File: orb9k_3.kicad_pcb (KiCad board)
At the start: 2 copper layers, 49.3 x 33 mm, 14 parts, among them IC2 MAX3232, J1 DB9-PowerDTRRTS, U2 SeeeduinoXIAO, U4 TC1240A

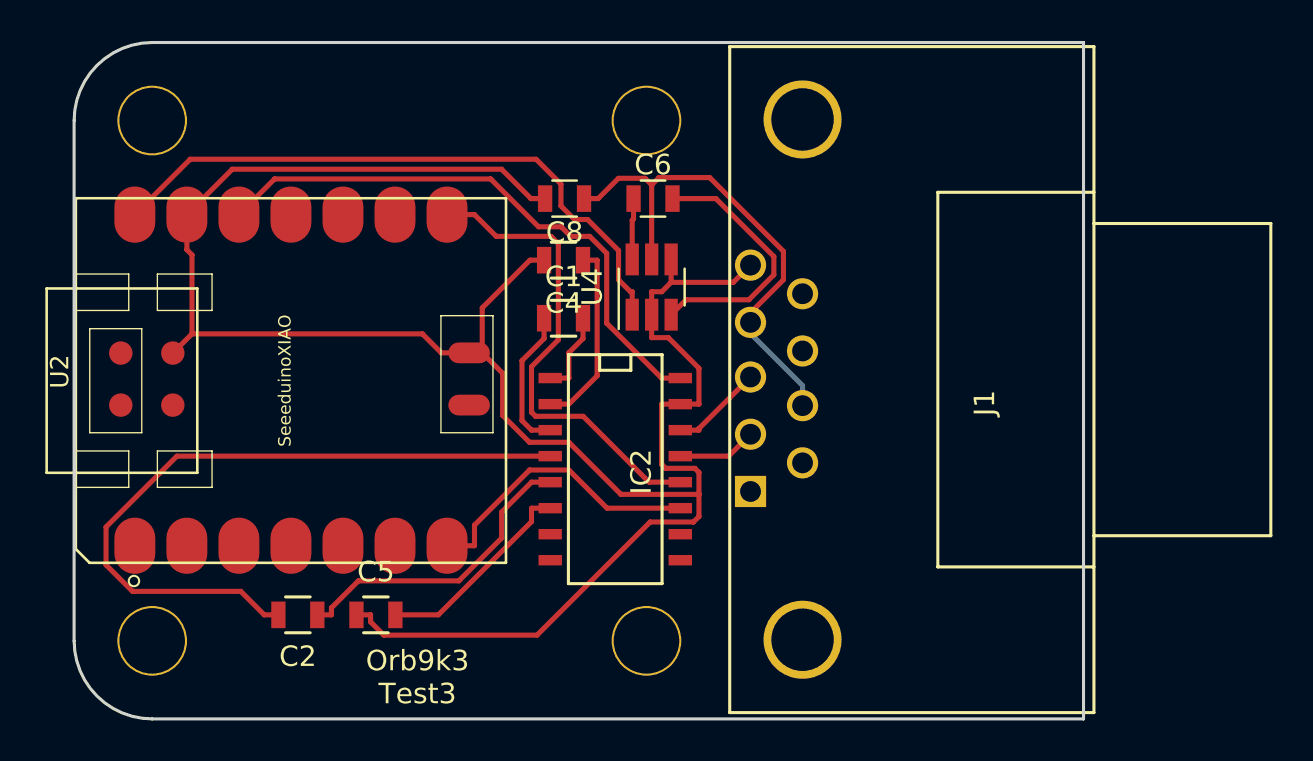
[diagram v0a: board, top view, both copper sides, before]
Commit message: Updates to orb9k_3
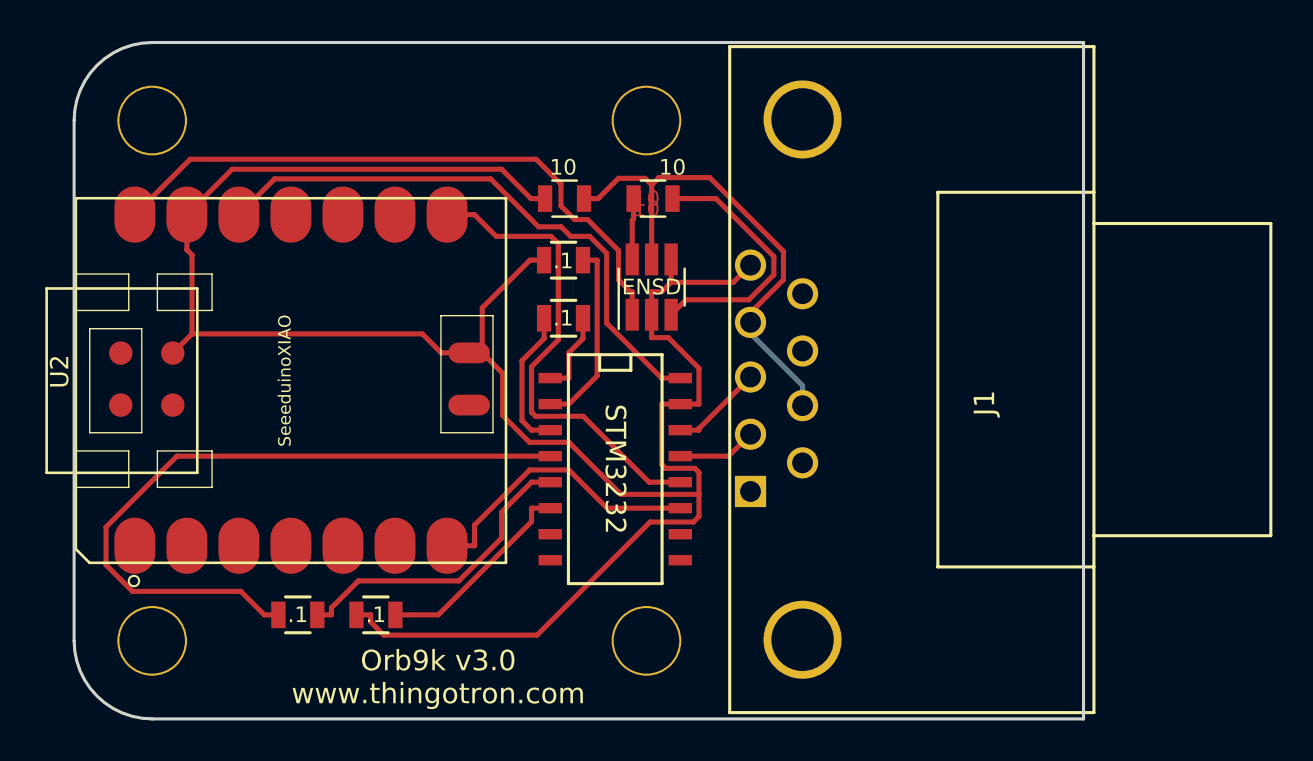
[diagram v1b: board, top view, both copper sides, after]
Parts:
- renumbered C1 to .1, C2 to .1, C4 to .1, C5 to .1, C8 to 10, C6 to 10, U4 to ENSD, IC2 to STM3232
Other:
- board text added: "10"
- board text added: "Orb9k v3.0 www.thingotron.com"
- board text removed: "Orb9k3 Test3"
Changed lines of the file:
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@@
   (general
     (thickness 1.6)
-    (drawings 8)
+    (drawings 10)
     (tracks 146)
     (zones 0)
@@
     (0 F.Cu signal)
     (31 B.Cu signal)
-    (32 B.Adhes user)
-    (33 F.Adhes user)
+    (32 B.Adhes user hide)
+    (33 F.Adhes user hide)
     (34 B.Paste user)
     (35 F.Paste user)
@@
     (47 F.CrtYd user)
     (48 B.Fab user)
-    (49 F.Fab user)
+    (49 F.Fab user hide)
   )
   (setup
@@
     (visible_elements 7FFFFFFF)
     (pcbplotparams
-      (layerselection 0x010f8_80000001)
+      (layerselection 0x010f8_ffffffff)
       (usegerberextensions true)
       (usegerberattributes false)
@@
       (drillshape 0)
       (scaleselection 1)
-      (outputdirectory "../proto_orders/20170102/"))
+      (outputdirectory "../proto_orders/20200509/gerbers"))
   )
   (net 0 "")
@@
     (tags "resistor 0805")
     (attr smd)
-    (fp_text reference C1 (at 0 2.032 180) (layer F.SilkS)
-      (effects (font (size 1 1) (thickness 0.15)))
+    (fp_text reference .1 (at 0.016 2.794 180) (layer F.SilkS)
+      (effects (font (size 0.762 0.762) (thickness 0.1524)))
     )
     (fp_text value 0.1uf (at 0 2.1 180) (layer F.Fab)
@@
     (tags "resistor 0805")
     (attr smd)
-    (fp_text reference C2 (at 0 2.032 180) (layer F.SilkS)
-      (effects (font (size 1 1) (thickness 0.15)))
+    (fp_text reference .1 (at 0 0 180) (layer F.SilkS)
+      (effects (font (size 0.762 0.762) (thickness 0.1524)))
     )
     (fp_text value 0.1uf (at 0 2.1 180) (layer F.Fab)
@@
     (tags "resistor 0805")
     (attr smd)
-    (fp_text reference C4 (at 0 -2.1 180) (layer F.SilkS)
-      (effects (font (size 1 1) (thickness 0.15)))
+    (fp_text reference .1 (at 0.016 -2.8365 180) (layer F.SilkS)
+      (effects (font (size 0.762 0.762) (thickness 0.1524)))
     )
     (fp_text value 0.1uf (at 0 2.1 180) (layer F.Fab)
@@
     (tags "resistor 0805")
     (attr smd)
-    (fp_text reference C5 (at 0 -2.1) (layer F.SilkS)
-      (effects (font (size 1 1) (thickness 0.15)))
+    (fp_text reference .1 (at 0 0) (layer F.SilkS)
+      (effects (font (size 0.762 0.762) (thickness 0.1524)))
     )
     (fp_text value 0.1uf (at -0.508 -2.032) (layer F.Fab)
@@
     (tags "CMS SOJ")
     (attr smd)
-    (fp_text reference IC2 (at 0.127 -1.27 270) (layer F.SilkS)
+    (fp_text reference STM3232 (at 0 0 270 unlocked) (layer F.SilkS)
       (effects (font (size 1 1) (thickness 0.15)))
     )
@@
     (tags "resistor 0805")
     (attr smd)
-    (fp_text reference C8 (at 0 -1.65) (layer F.SilkS)
-      (effects (font (size 1 1) (thickness 0.15)))
+    (fp_text reference 10 (at 0.066 1.524) (layer F.SilkS)
+      (effects (font (size 0.762 0.762) (thickness 0.1524)))
     )
     (fp_text value 10uf (at 0 1.75) (layer F.Fab)
@@
     (tags "SOT-23-6 Handsoldering")
     (attr smd)
-    (fp_text reference U4 (at 0 -2.9 90) (layer F.SilkS)
-      (effects (font (size 1 1) (thickness 0.15)))
+    (fp_text reference ENSD (at 0 0 180) (layer F.SilkS)
+      (effects (font (size 0.762 0.762) (thickness 0.1524)))
     )
     (fp_text value TC1240A (at 0 2.9 90) (layer F.Fab)
@@
     (tags "resistor 0805")
     (attr smd)
-    (fp_text reference C6 (at 0 -1.65) (layer F.SilkS)
-      (effects (font (size 1 1) (thickness 0.15)))
+    (fp_text reference 10 (at 0.95 -1.524) (layer F.SilkS)
+      (effects (font (size 0.762 0.762) (thickness 0.15)))
     )
     (fp_text value 10uf (at 0 1.75) (layer F.Fab)
@@
     )
   )
-  (gr_text "Orb9k3\nTest3" (at 61.764 106.988) (layer F.SilkS)
+  (gr_text 10 (at 72.94 84.128) (layer F.Cu)
+    (effects (font (size 0.762 0.762) (thickness 0.1905)))
+  )
+  (gr_text 10 (at 72.94 83.62) (layer F.Cu)
+    (effects (font (size 0.762 0.762) (thickness 0.1905)))
+  )
+  (gr_text "Orb9k v3.0\nwww.thingotron.com" (at 62.78 106.988) (layer F.SilkS)
     (effects (font (size 1 1) (thickness 0.2)))
   )
